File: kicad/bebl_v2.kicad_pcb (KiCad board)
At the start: 2 copper layers, 80 x 39 mm, 73 parts, among them P1 ISP, P10 LED_DRL, P11 DRV_LED, P12 CHG_LED, P13 LED_CHG, P2 FTDI, P3 LiPo, P4 USB-Micro, P8 DRL_LED, P9 LED_DRV, SW1 RST, SW2 MODE, U1 ATMEGA328, U2 FAN5346, U3 ADXL345, U4 MCP73831, U5 TPS61221DCK, X1 8MHz

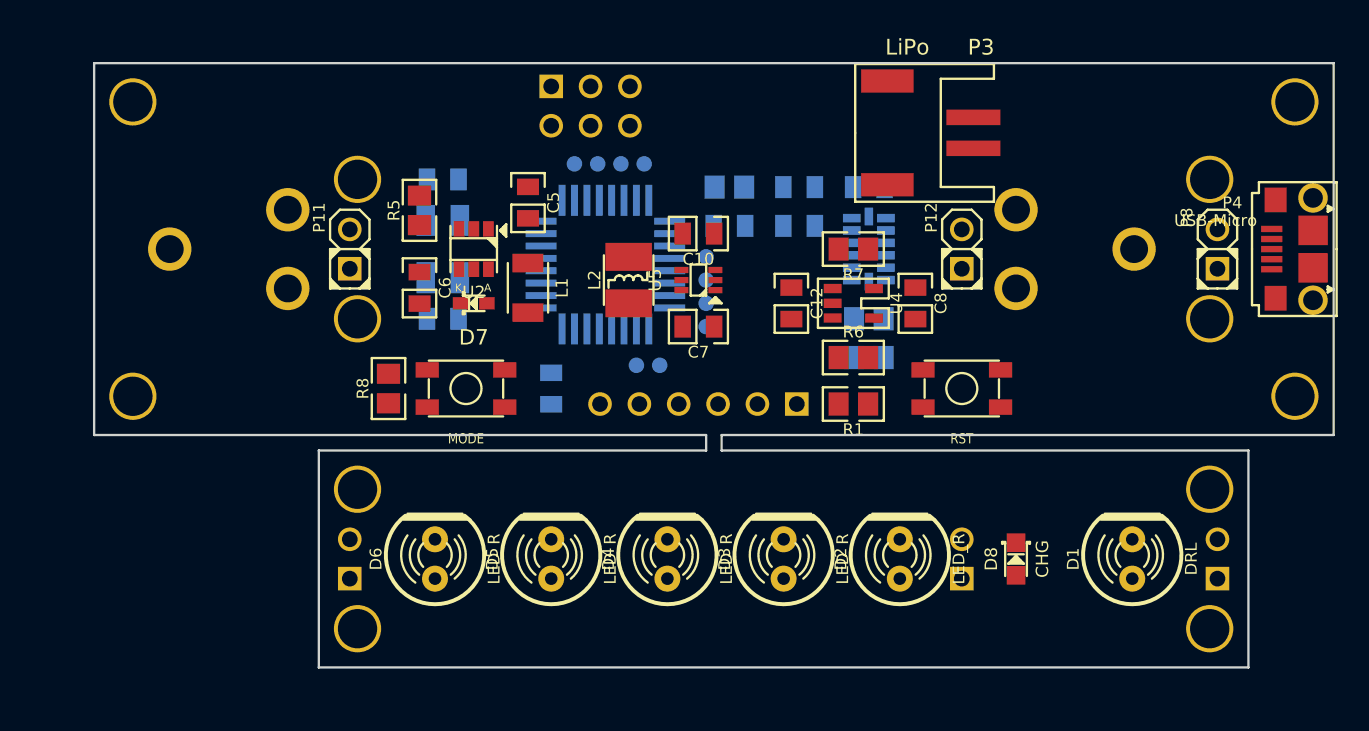
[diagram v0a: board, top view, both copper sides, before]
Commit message: bebl_v2 track layout, work in progress
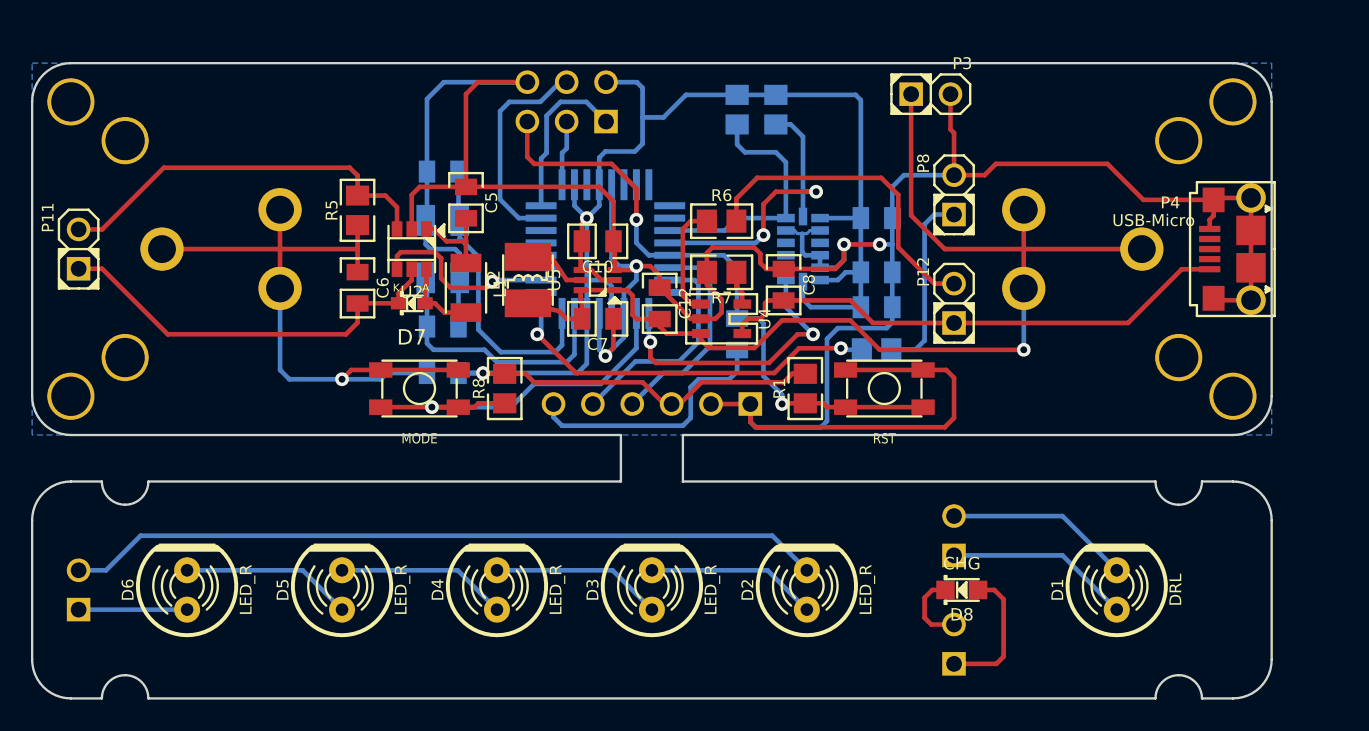
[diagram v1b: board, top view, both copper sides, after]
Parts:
- removed B1, B10, B11, B12, B13, B2, B3, B4, B5, B6: I/O, bebl_v2_pretty:breakout_smd
- removed SC10, SC11, SC12, SC9: SCREW, bebl_v2_pretty:screw_3mm
- P3: footprint bebl_v2_pretty:CONN_JST-2_SMD -> bebl_v2_pretty:pin_strip_2
- moved C3 20.8 mm to (60.5, 58.0), turned to 0 degrees
- moved R2 18.1 mm to (79.5, 41.0), turned to 90 degrees
- moved P9 17.6 mm to (37.0, 72.0)
- moved P11 17.5 mm to (37.0, 50.0)
- moved P8 17.4 mm to (93.5, 46.5)
- moved P10 17.1 mm to (93.5, 68.5)
- moved D6 16.1 mm to (44.0, 72.0)
- moved SC5 15.2 mm to (40.0, 57.0)
- moved SC6 15.2 mm to (40.0, 43.0)
- moved R3 14.8 mm to (82.0, 41.0), turned to 90 degrees
- moved R4 14.2 mm to (88.5, 56.5)
- moved D5 13.6 mm to (54.0, 72.0)
- moved C4 12.5 mm to (79.5, 55.5)
- moved R6 12.2 mm to (78.5, 48.2)
- moved D4 11.2 mm to (64.0, 72.0)
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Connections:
- P4 pad 2: (no net) -> Net-(P4-Pad2)
- P4 pad 3: (no net) -> Net-(P4-Pad3)
- P4 pad 4: (no net) -> Net-(P4-Pad4)
- U1 pad 1: /ACL_INT2 -> /ACL_INT1
- U1 pad 32: /ACL_INT1 -> /ACL_INT2
- U3 pad 10: (no net) -> Net-(U3-Pad10)
- U3 pad 11: (no net) -> Net-(U3-Pad11)
- U3 pad 3: (no net) -> Net-(U3-Pad3)
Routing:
- net GND: track 0.00 -> 245.7 mm, vias 0 -> 5
- net +3.3V: track 0.00 -> 106.4 mm, vias 0 -> 2
- net /BAT: track 0.00 -> 71.2 mm, vias 0 -> 1
- net /CATH: track 0.00 -> 48.8 mm
- net /RESET: track 0.00 -> 40.8 mm, vias 0 -> 2
- net /VUSB: track 0.00 -> 33.8 mm
- net /MODE: track 0.00 -> 26.8 mm, vias 0 -> 1
- net /LED_A: track 0.00 -> 26.5 mm
- net /DRL_PWM: track 0.00 -> 25.5 mm, vias 0 -> 2
- net /LED_K: track 0.00 -> 25.4 mm
- net Net-(P12-Pad2): track 0.00 -> 20.9 mm
- net /SCL: track 0.00 -> 20.1 mm, vias 0 -> 2
- net /PB7: track 0.00 -> 19.0 mm
- net /ACL_INT1: track 0.00 -> 18.5 mm, vias 0 -> 2
- net /PB6: track 0.00 -> 17.1 mm
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- added copper zone on B.Cu, net GND
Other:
- board size 80 x 39 mm -> 80 x 41 mm
- net class 0.2mm added: clearance 0.2, trace_width 0.2, via_dia 0.889, via_drill 0.635
- net class Default: clearance 0.254 -> 0.25; trace_width 0.254 -> 0.3
- rule trace_clearance: 0.254 -> 0.25
- rule trace_min: 0.254 -> 0.2
